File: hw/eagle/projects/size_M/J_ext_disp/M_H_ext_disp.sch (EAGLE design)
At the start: 18 parts, among them U1 CP2104-F03-GM

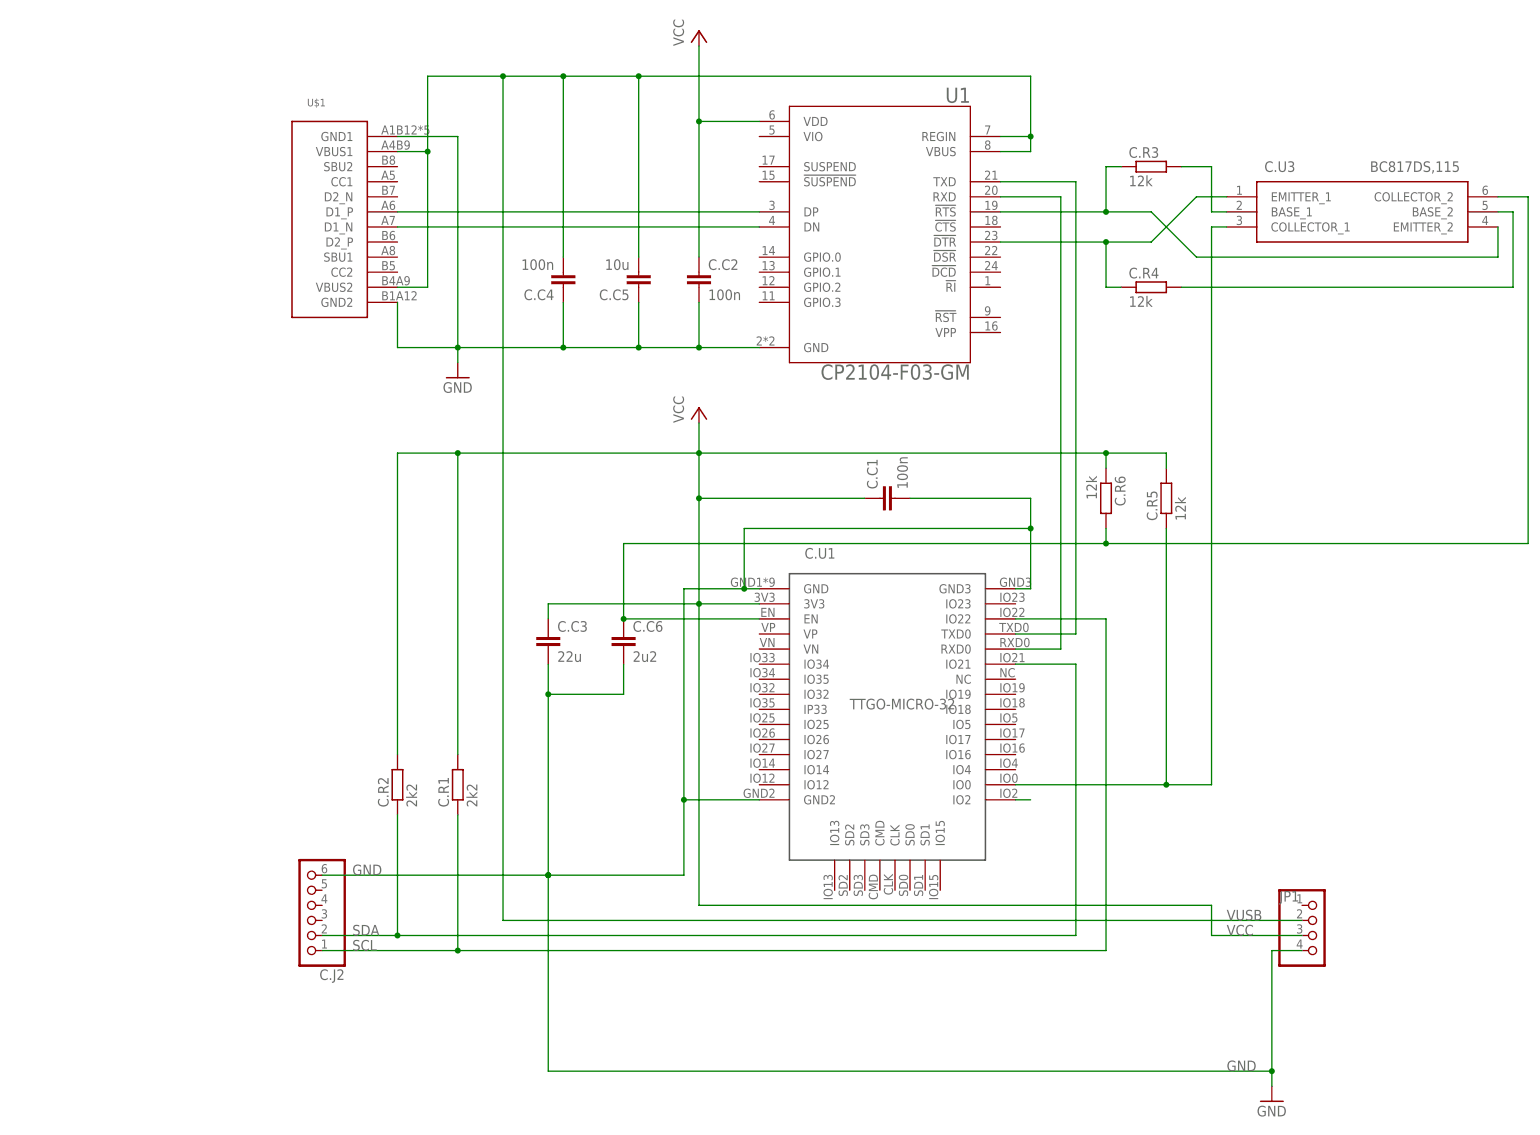
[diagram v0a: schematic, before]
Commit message: pcb M.1 -not finished
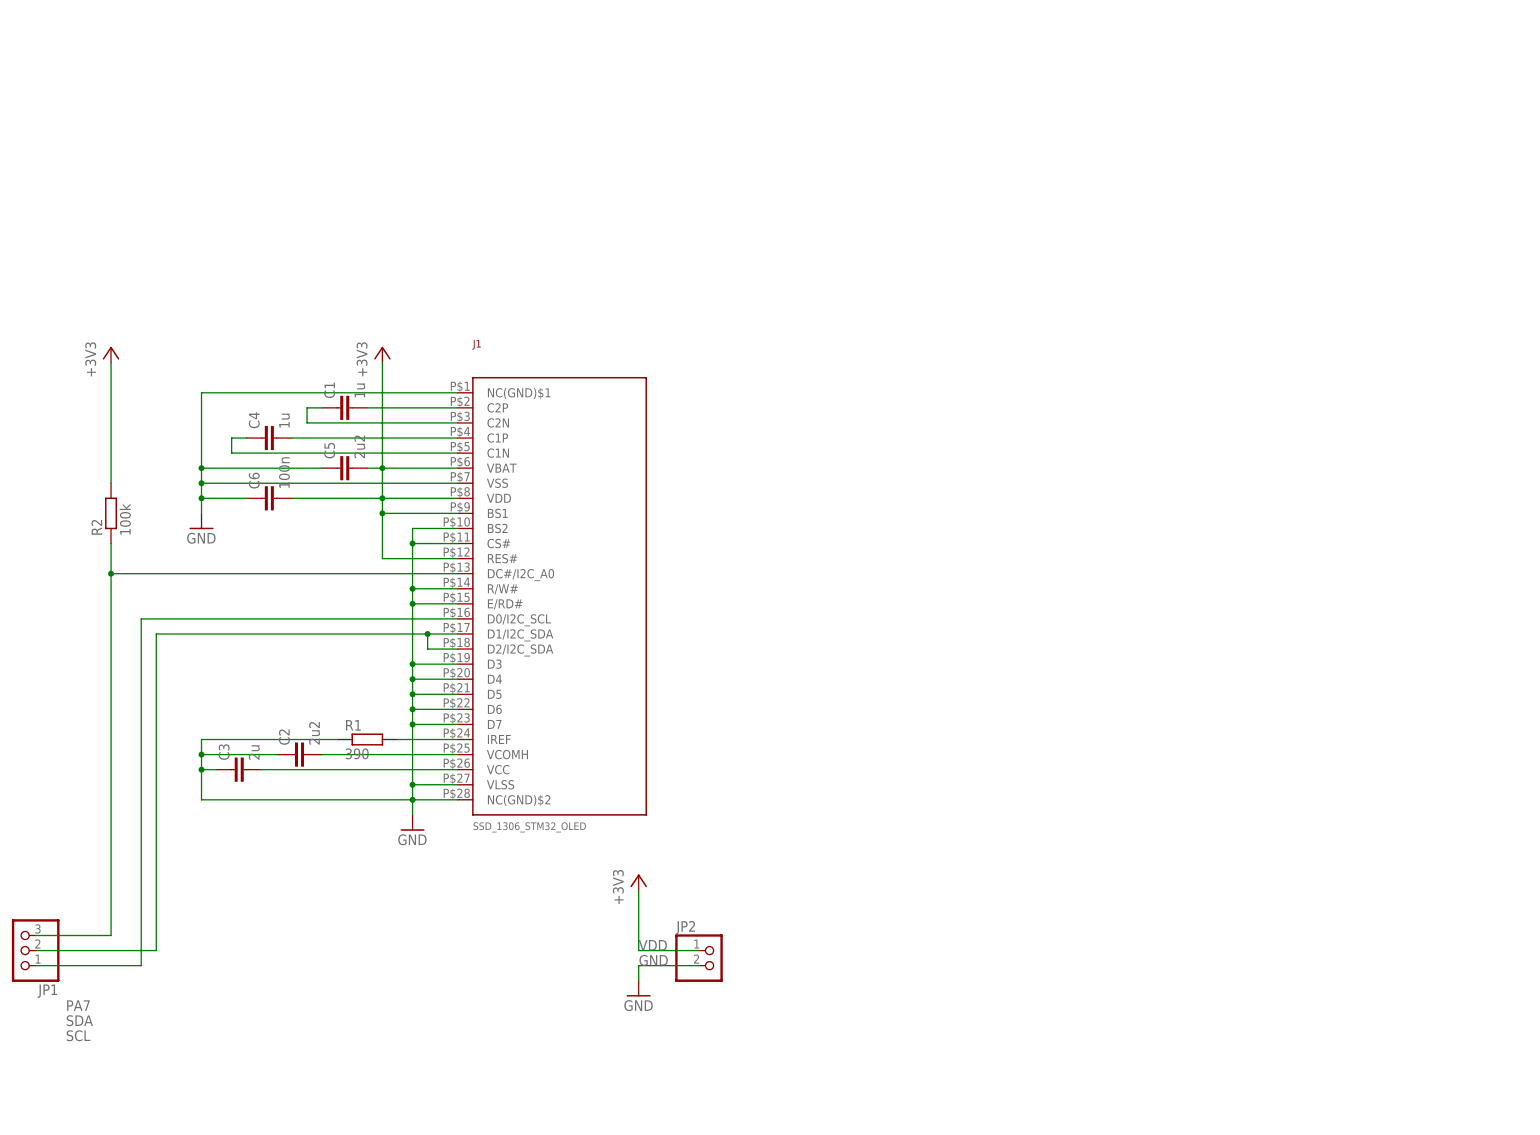
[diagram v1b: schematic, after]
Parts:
- removed C.C1, C.C2, C.C4: 100n, rcl:C-EUC0603
- removed C.C3: 22u, rcl:C-EUC0805
- removed C.C5: 10u, rcl:C-EUC0603
- removed C.C6: 2u2, rcl:C-EUC0603
- removed C.J2: (no value), pinhead2:PINHD-1X6
- removed C.R1, C.R2: 2k2, rcl:R-EU_R0603
- removed C.R3, C.R4, C.R5, C.R6: 12k, rcl:R-EU_R0603
- removed C.U1: TTGO-MICRO-32, hugo:TTGO-MICRO-32
- removed C.U3: BC817DS,115, SamacSys_Parts:BC817DS,115
- removed U$1: USB-C, hugo:USB-C
- removed U1: CP2104-F03-GM, CP2104:CP2104-F03-GM
- added C1, C4: 1u, rcl:C-EUC0603
- added C2, C5: 2u2, rcl:C-EUC0603
- added C3: 2u, rcl:C-EUC0603
- added C6: 100n, rcl:C-EUC0603
- added J1: SSD_1306_STM32_OLED, hugo:SSD_1306_STM32_OLED
- added JP2: (no value), pinhead2:PINHD-1X2
- added R1: 390, rcl:R-EU_R0603
- added R2: 100k, rcl:R-EU_R0603
- JP1: device pinhead2:PINHD-1X4 -> pinhead2:PINHD-1X3
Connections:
- removed net N$11: C.C6.1, C.R6.2, C.U1.EN, C.U3.COLLECTOR_2
- removed net N$13: C.U1.IO2
- removed net N$2: U$1.D1_P, U1.DP
- removed net RX: C.U1.RXD0, U1.RXD
- removed net TX: C.U1.TXD0, U1.TXD
- removed net VCC: C.C1.1, C.C2.1, C.C3.1, C.R1.2, C.R2.2, C.R5.2, C.R6.1, C.U1.3V3, JP1.3, U1.VDD
- removed net VUSB: C.C4.2, C.C5.2, JP1.2, U$1.VBUS1, U$1.VBUS2, U1.REGIN, U1.VBUS
- new net N$3: C3.2, J1.VCC
- new net PA7: J1.DC#/I2C_A0, JP1.3, R2.1
- new net VDD: C5.2, C6.2, J1.BS1, J1.RES#, J1.VBAT, J1.VDD, JP2.1, R2.2
- net GND: now also C2.1, C3.1, C5.1, C6.1, J1.BS2, J1.CS#, J1.D3, J1.D4, J1.D5, J1.D6, J1.D7, J1.E/RD#, J1.NC(GND)$1, J1.NC(GND)$2, J1.R/W#, J1.VLSS, J1.VSS, JP2.2, R1.1; no longer C.C1.2, C.C2.2, C.C3.2, C.C4.1, C.C5.1, C.C6.2, C.J2.6, C.U1.GND, C.U1.GND2, C.U1.GND3, JP1.4, U$1.GND1, U$1.GND2, U1.GND
- net N$1: now also J1.IREF, R1.2; no longer U$1.D1_N, U1.DN
- net N$10: now also C4.1, J1.C1N; no longer C.R5.1, C.U1.IO0, C.U3.COLLECTOR_1
- net N$5: now also C2.2, J1.VCOMH; no longer C.R4.2, C.U3.BASE_2
- net N$7: now also C1.2, J1.C2P; no longer C.R3.2, C.U3.BASE_1
- net N$8: now also C1.1, J1.C2N; no longer C.R3.1, C.U3.EMITTER_2, U1.!RTS
- net N$9: now also C4.2, J1.C1P; no longer C.R4.1, C.U3.EMITTER_1, U1.!DTR
- net SCL: now also J1.D0/I2C_SCL, JP1.1; no longer C.J2.1, C.R1.1, C.U1.IO22
- net SDA: now also J1.D1/I2C_SDA, J1.D2/I2C_SDA, JP1.2; no longer C.J2.2, C.R2.1, C.U1.IO21
